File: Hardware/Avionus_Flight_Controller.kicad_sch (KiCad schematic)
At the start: 0 parts

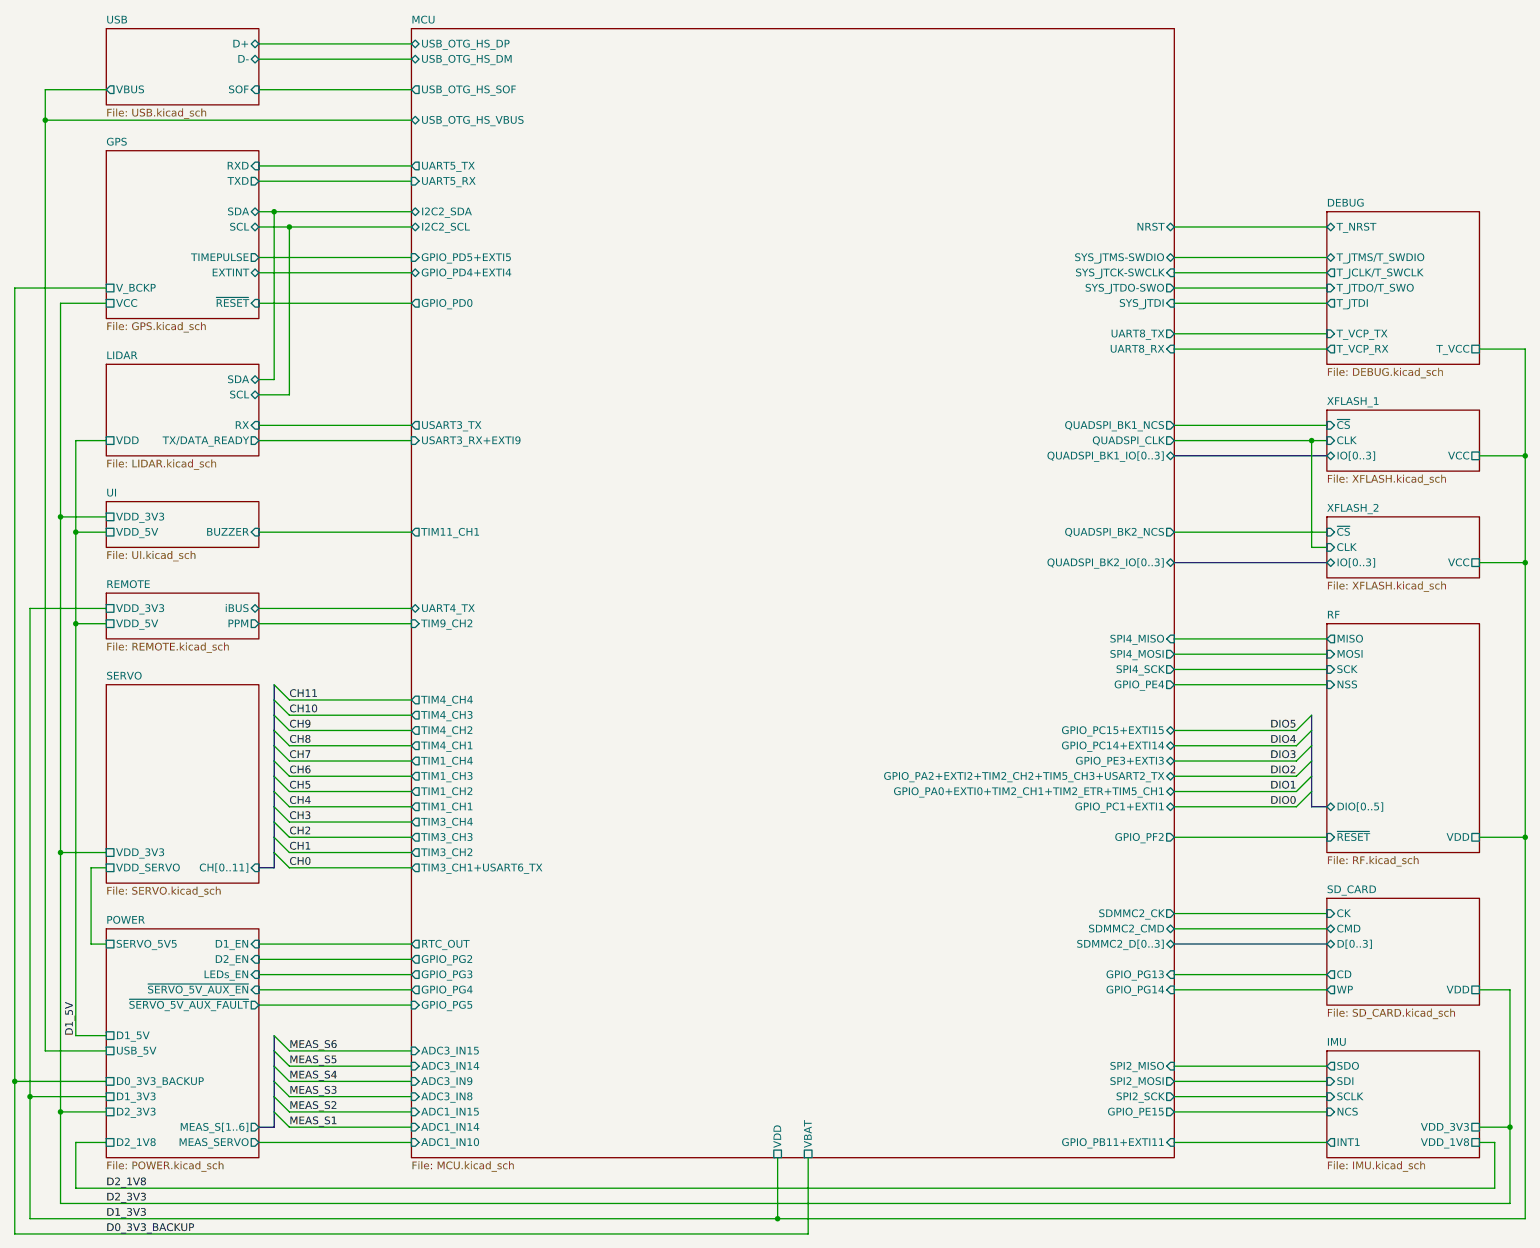
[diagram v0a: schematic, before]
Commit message: Checkpoint
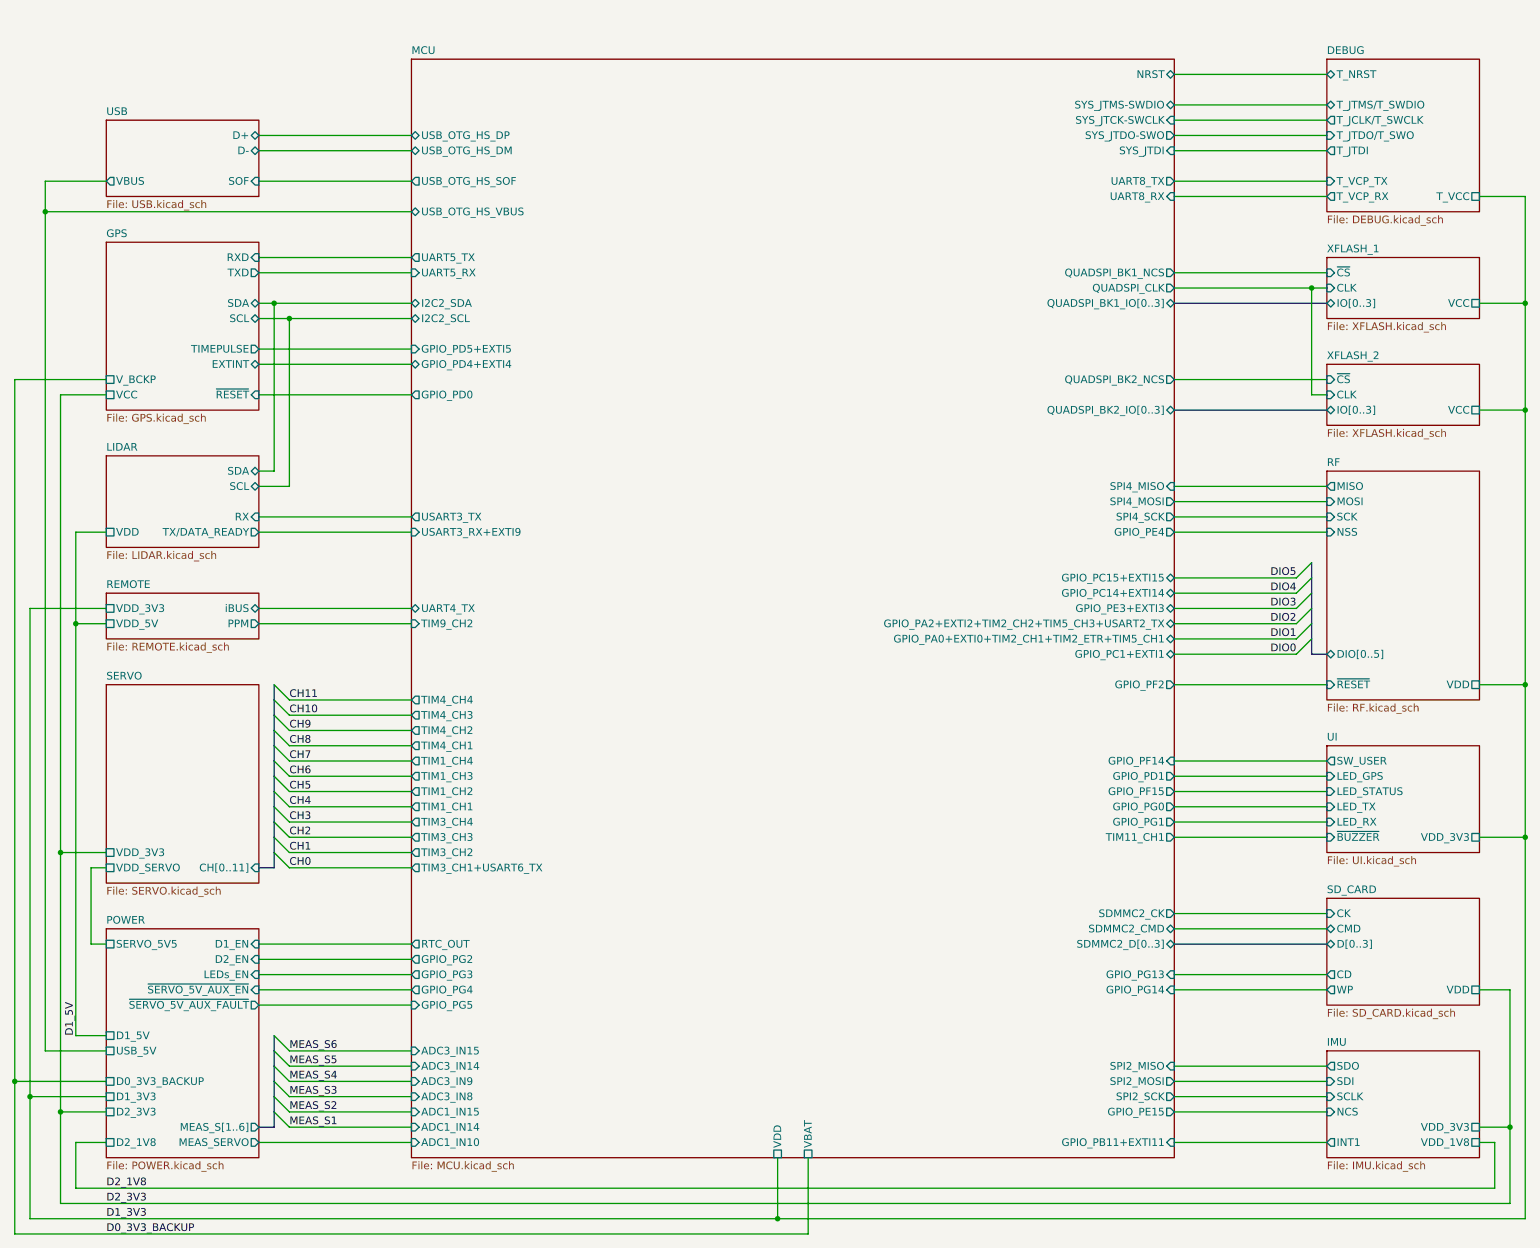
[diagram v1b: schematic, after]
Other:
- sheet MCU ports: added GPIO_PD1, GPIO_PF14, GPIO_PF15, GPIO_PG0, GPIO_PG1; removed none
- sheet UI ports: added LED_GPS, LED_RX, LED_STATUS, LED_TX, SW_USER, ~{BUZZER}; removed BUZZER, VDD_5V
